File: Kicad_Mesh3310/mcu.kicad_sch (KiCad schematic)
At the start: 41 parts, among them U12 ZD25WQ16CTIGT, U13 NRF52840-QIAA-R, X2 S201632M10PF10PPM 32MHz, X4 32.768KHz

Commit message: Start of routing
Component placing and start off routing
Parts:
- C36: footprint Capacitor_SMD:C_0603_1608Metric -> Capacitor_SMD:C_0402_1005Metric
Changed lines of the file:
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@@
 			)
 		)
-		(property "Footprint" "Capacitor_SMD:C_0603_1608Metric"
+		(property "Footprint" "Capacitor_SMD:C_0402_1005Metric"
 			(at 194.6148 71.12 0)
 			(effects

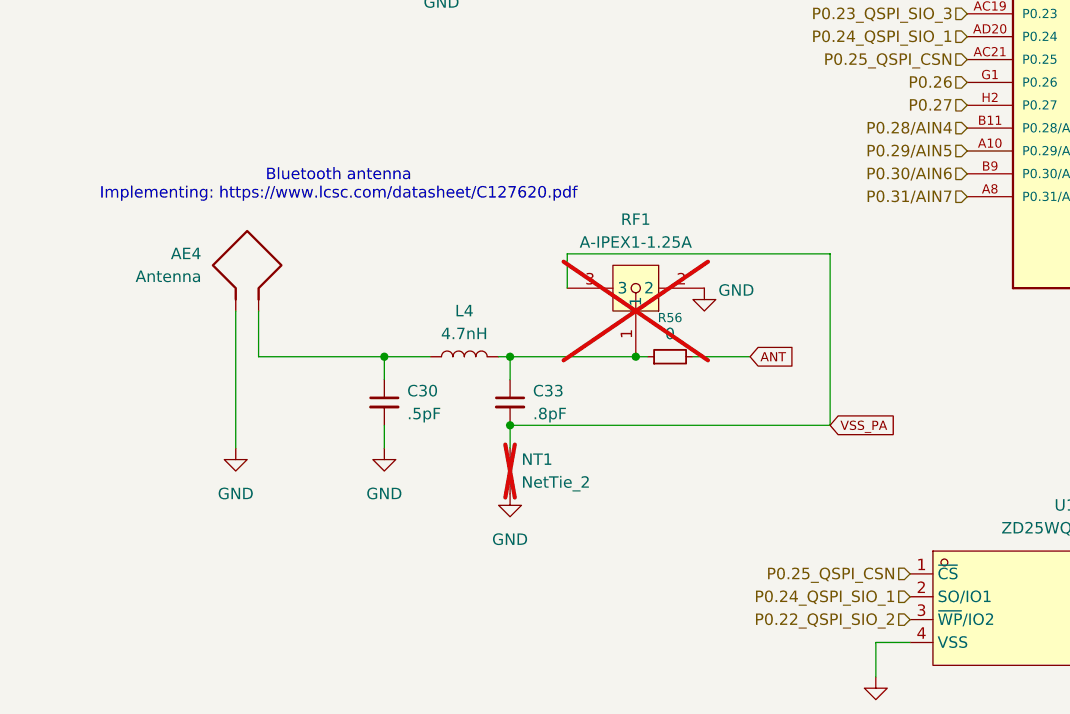
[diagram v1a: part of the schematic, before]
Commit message: RF designing
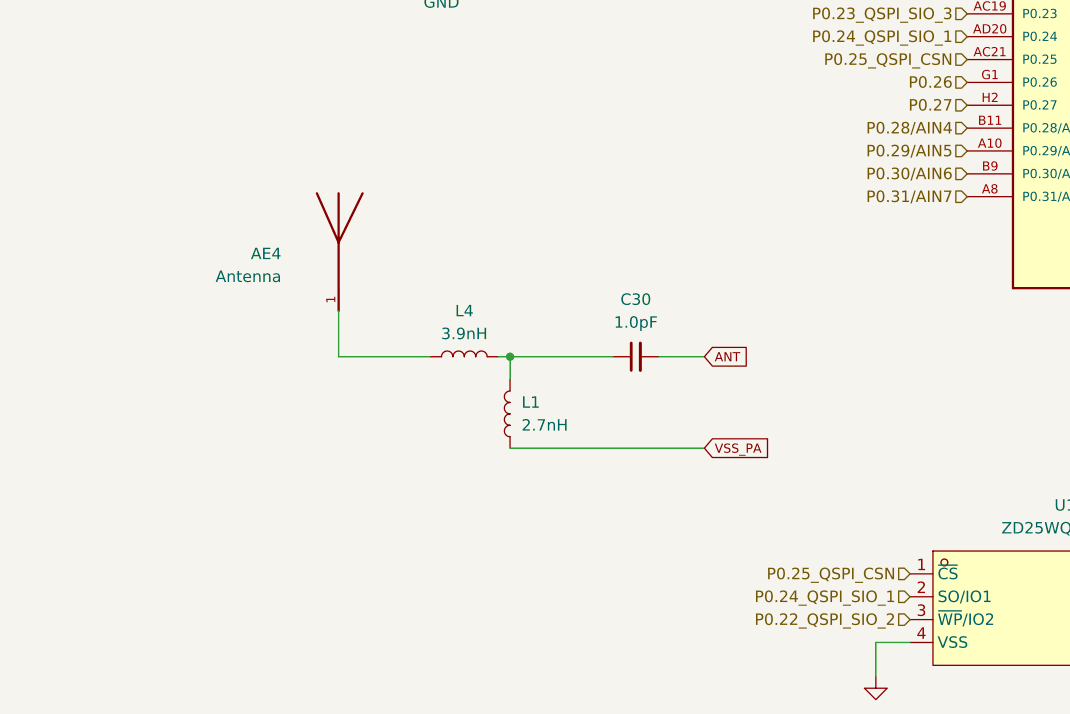
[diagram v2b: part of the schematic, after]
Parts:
- removed C33: .8pF, Capacitor_SMD:C_0402_1005Metric, symbol Device:C_Small
- removed NT1: NetTie_2, NetTie:NetTie-2_SMD_Pad0.5mm, symbol Device:NetTie_2
- removed R56: 0, Resistor_SMD:R_0402_1005Metric, symbol Device:R_Small
- removed RF1: A-IPEX1-1.25A, mesh3310_footprints:IPEX-SMD_3P-L2.6-W2.6-LS3.0_RF1200001R, symbol lcsc:A-IPEX1-1.25A
- added L1: 2.7nH, Inductor_SMD:L_0402_1005Metric, symbol Device:L
- AE4: footprint RF_Antenna:Texas_SWRA117D_2.4GHz_Right -> mesh3310_footprints:XCVR_2450AT18A0100001E; symbol Device:Antenna_Loop -> 2450AT18A0100001E:2450AT18A0100001E; Availability (none) -> In Stock; Check_prices (none) -> https://www.snapeda.com/parts/2450AT18A0100001E/Johanson/vi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; Description_1 (none) -> RF ANTENNA Chip Solder Surface Mount; MANUFACTURER (none) -> Johanson Technology; MAXIMUM_PACKAGE_HEIGHT (none) -> 1.40 mm; MF (none) -> Johanson Technology Inc.; MP (none) -> 2450AT18A0100001E; PARTREV (none) -> 4.0; Package (none) -> None; Price (none) -> None; Purchase-URL (none) -> https://www.snapeda.com/api/url_track_click_mouser/?unipart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; STANDARD (none) -> Manufacturer recommendations; SnapEDA_Link (none) -> https://www.snapeda.com/parts/2450AT18A0100001E/Johanson/vi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; now in the parts list
- C30: value .5pF -> 1.0pF
- L4: value 4.7nH -> 3.9nH
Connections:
- net ANT: now also C30.2
- net GND: no longer AE4.2, C30.2
- net VSS_PA: now also L1.1
- net at AE4.1, L4.1: no longer C30.1
- net at L4.2: now also C30.1, L1.2
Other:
- note removed: "Bluetooth antenna Implementing: https://www.lcsc.com/datasheet/C127620.pdf"
- moved on the sheet: C30

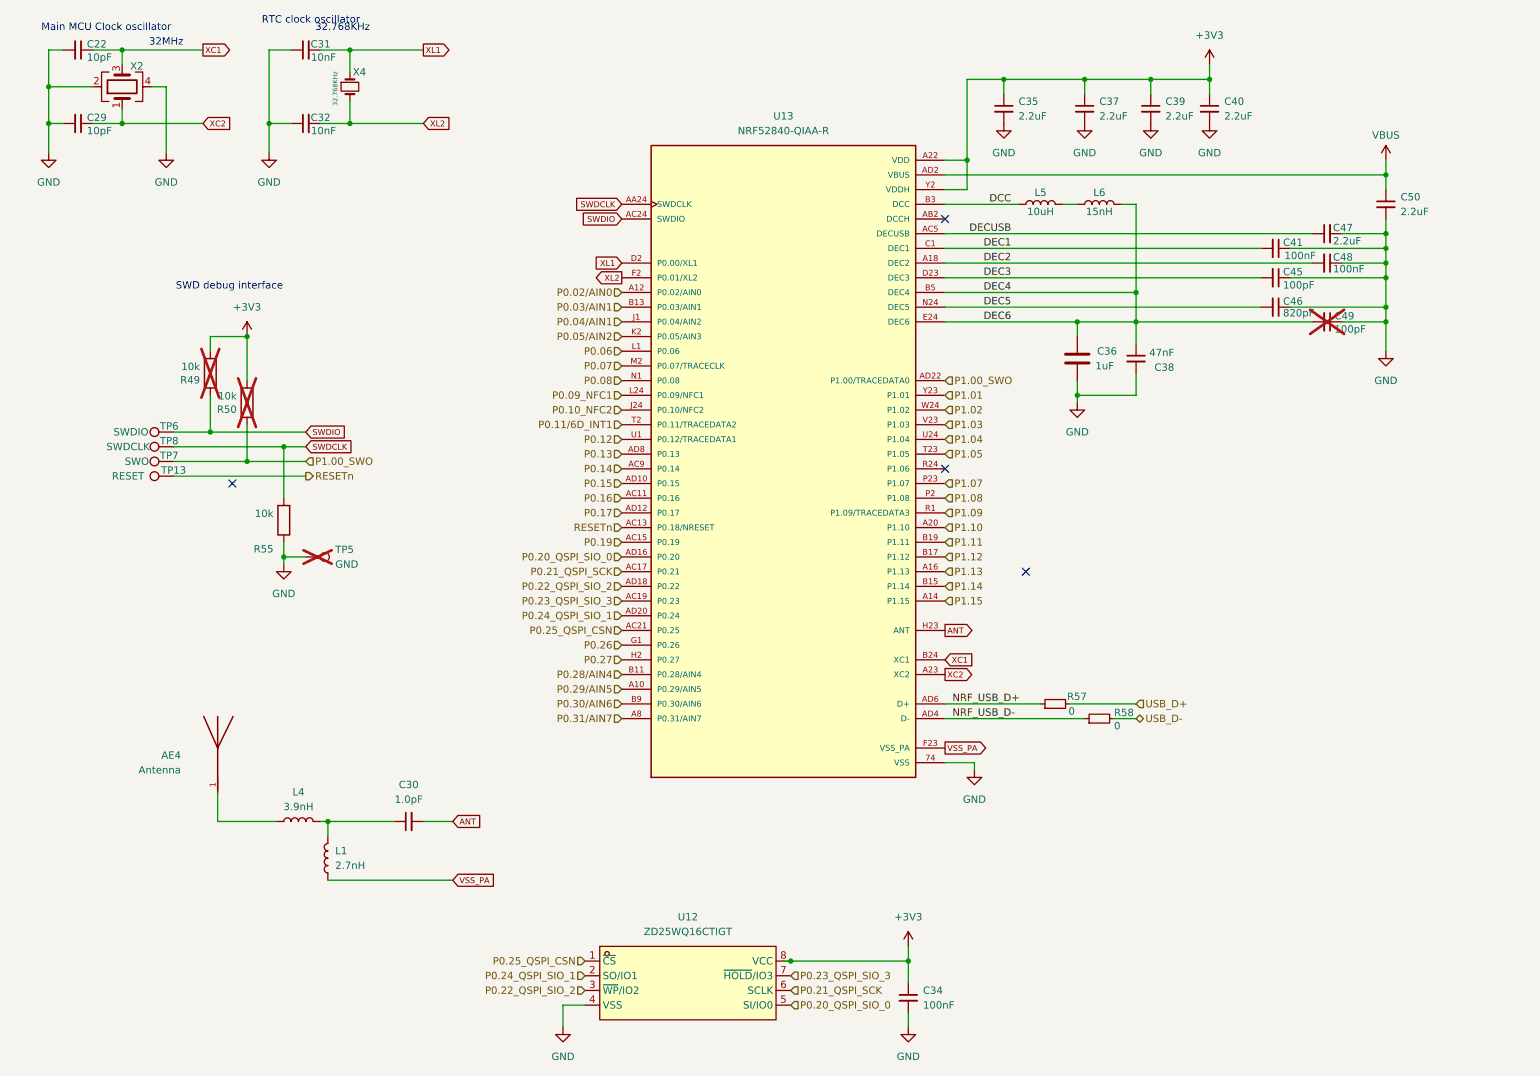
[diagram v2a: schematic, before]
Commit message: cleanup
schematic cleanup
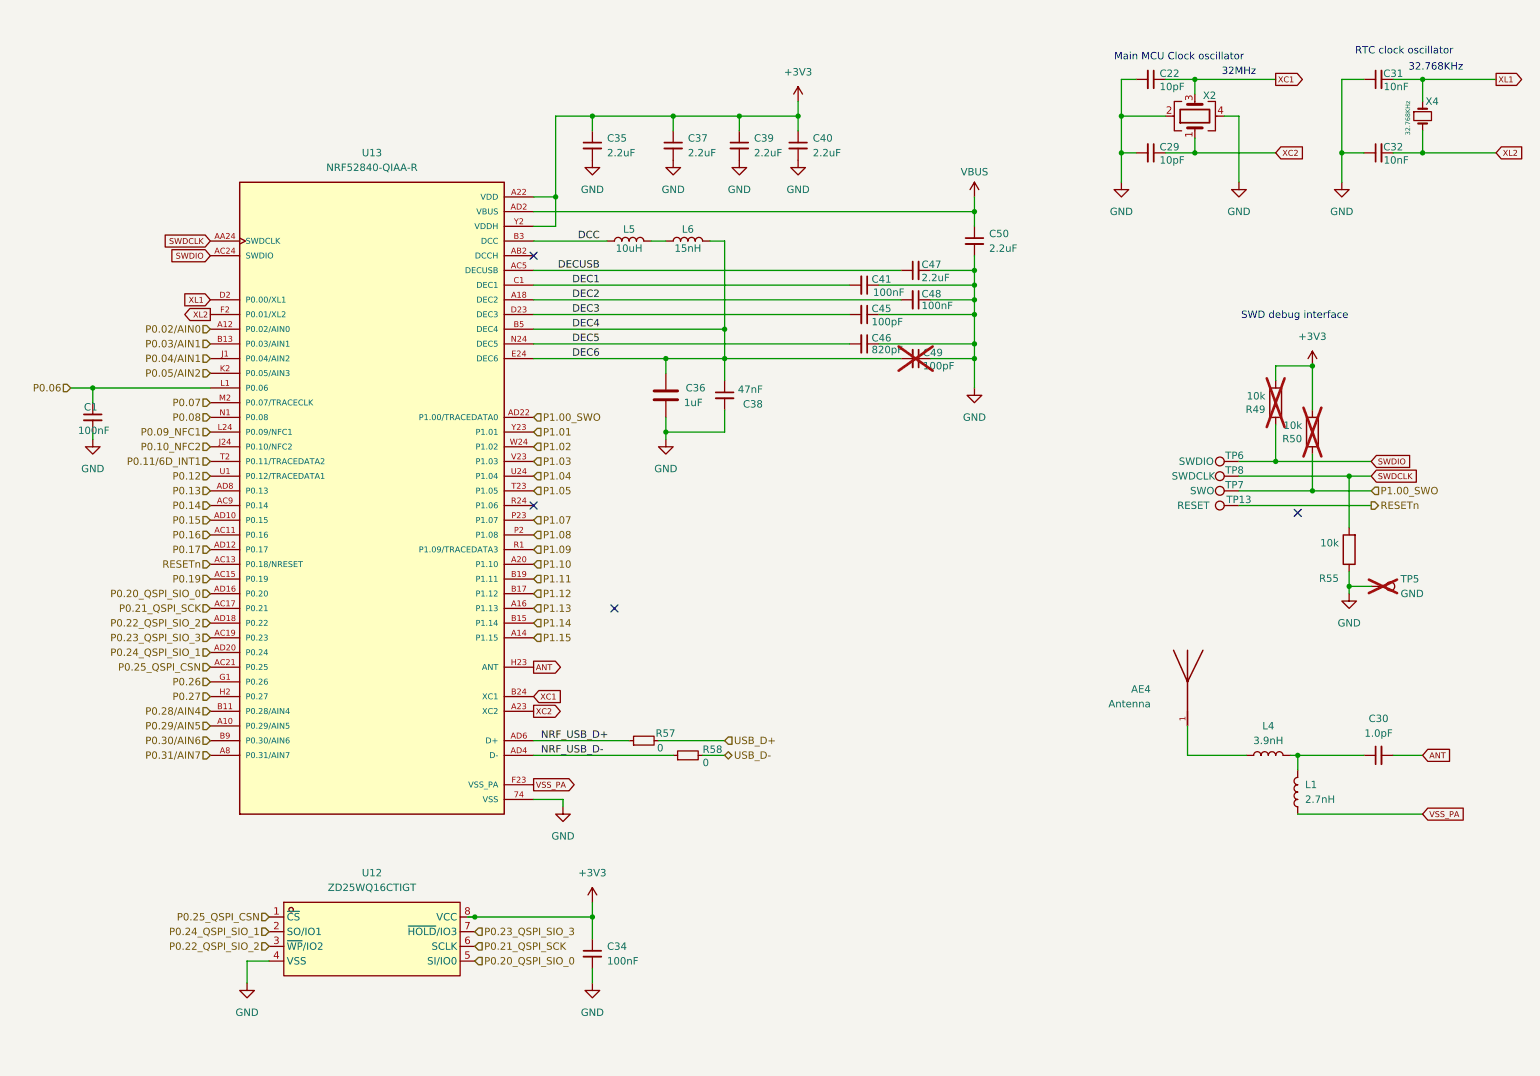
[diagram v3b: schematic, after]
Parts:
- added C1: 100nF, Capacitor_SMD:C_0402_1005Metric, symbol Device:C_Small
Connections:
- net GND: now also C1.2
- net P0.06: now also C1.1
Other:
- moved on the sheet: AE4, C22, C29, C30, C31, C32, C34, C35, C36, C37, C38, C39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
